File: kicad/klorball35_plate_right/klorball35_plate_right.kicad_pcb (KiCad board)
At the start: 2 copper layers, 138.1 x 106.1 mm, 8 parts

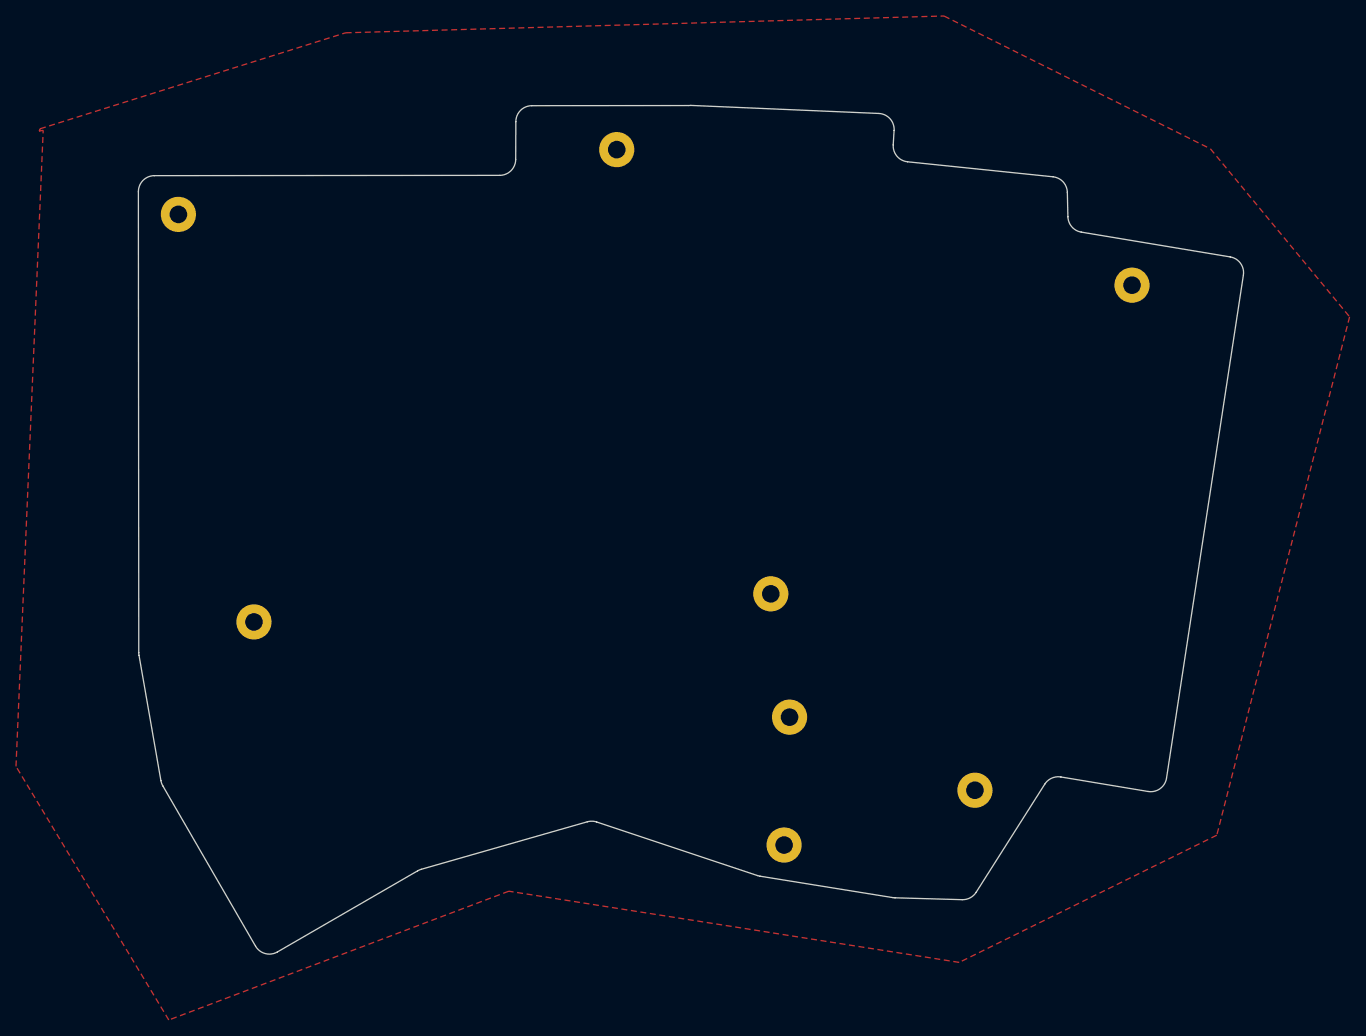
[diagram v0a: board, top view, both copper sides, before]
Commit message: Wrapping up, re-organizing.  Final gerbers and designs
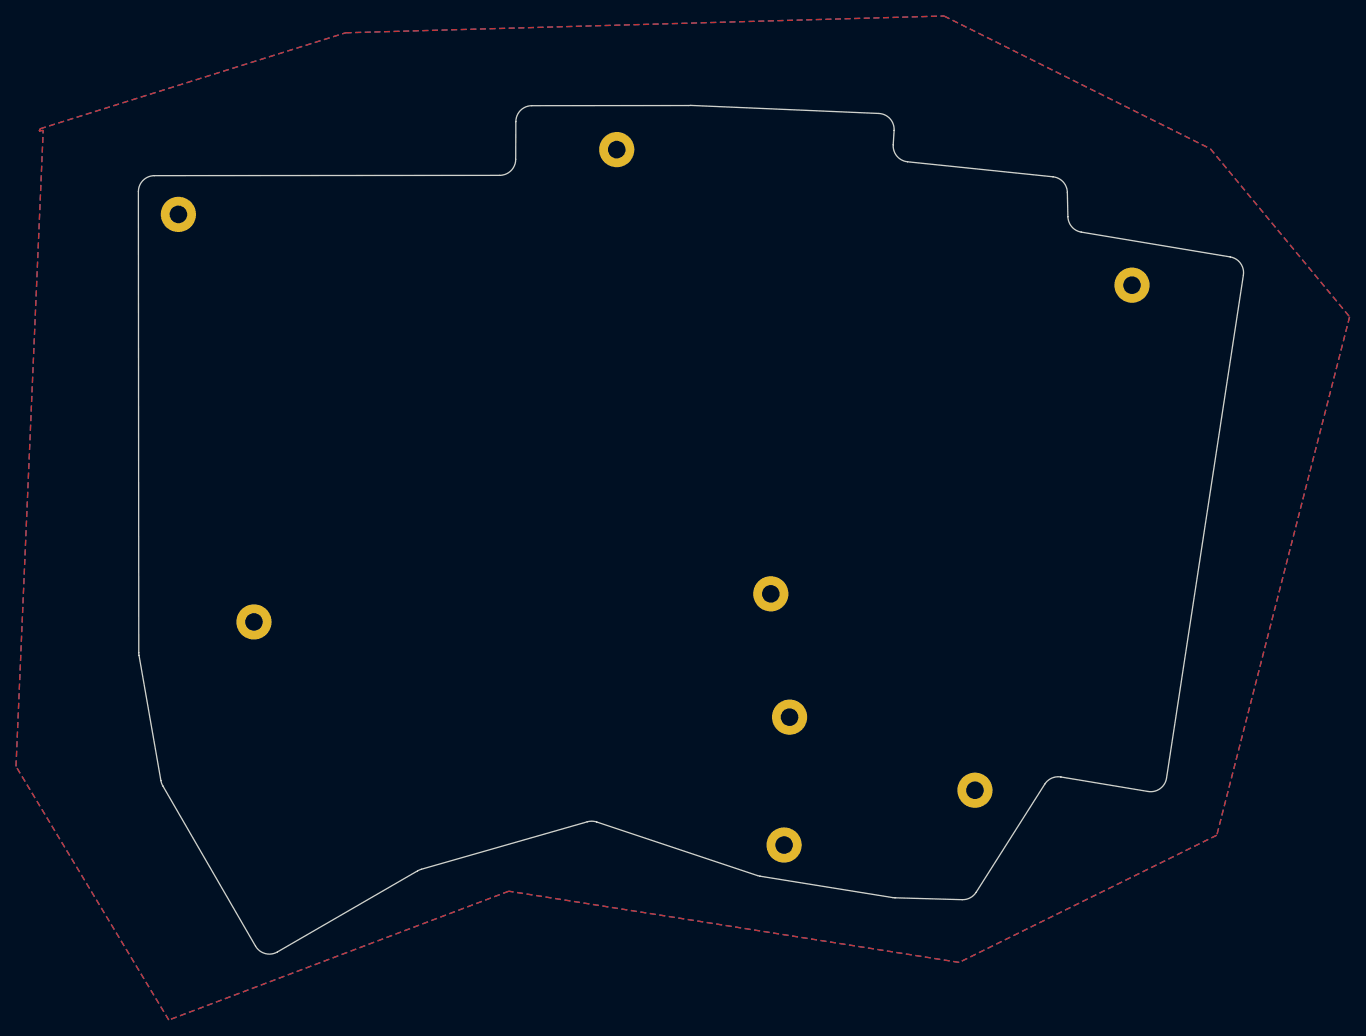
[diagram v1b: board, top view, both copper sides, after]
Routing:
- added copper zone on B.Cu, net (none)
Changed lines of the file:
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@@
 		(0 "F.Cu" signal)
 		(2 "B.Cu" signal)
-		(9 "F.Adhes" user)
-		(11 "B.Adhes" user)
+		(9 "F.Adhes" user "F.Adhesive")
+		(11 "B.Adhes" user "B.Adhesive")
 		(13 "F.Paste" user)
 		(15 "B.Paste" user)
-		(5 "F.SilkS" user)
-		(7 "B.SilkS" user)
+		(5 "F.SilkS" user "F.Silkscreen")
+		(7 "B.SilkS" user "B.Silkscreen")
 		(1 "F.Mask" user)
 		(3 "B.Mask" user)
-		(17 "Dwgs.User" user)
-		(19 "Cmts.User" user)
-		(21 "Eco1.User" user)
-		(23 "Eco2.User" user)
+		(17 "Dwgs.User" user "User.Drawings")
+		(19 "Cmts.User" user "User.Comments")
+		(21 "Eco1.User" user "User.Eco1")
+		(23 "Eco2.User" user "User.Eco2")
 		(25 "Edge.Cuts" user)
 		(27 "Margin" user)
-		(31 "F.CrtYd" user)
-		(29 "B.CrtYd" user)
+		(31 "F.CrtYd" user "F.Courtyard")
+		(29 "B.CrtYd" user "B.Courtyard")
 		(35 "F.Fab" user)
 		(33 "B.Fab" user)
@@
 		(net 0)
 		(net_name "")
-		(layer "F.Cu")
+		(layers "F.Cu" "B.Cu")
 		(hatch edge 0.5)
 		(connect_pads
@@
 			(pts
 				(xy 132.3 88.3) (xy 170.5 76.3) (xy 245.3 74.2) (xy 278.6 90.8) (xy 296 111.8) (xy 279.4 176.6)
-				(xy 247.2 192.5) (xy 190.9 183.6) (xy 148.4 199.7) (xy 129.3 168) (xy 132.7 88.5) (xy 132.7 88.5)
-				(xy 132.6 88.5) (xy 132.2 88.6)
-			)
-		)
+				(xy 247.2 192.5) (xy 190.9 183.6) (xy 148.4 199.7) (xy 129.3 168) (xy 132.7 88.5) (xy 132.6 88.5)
+				(xy 132.2 88.6)
+			)
+		)
